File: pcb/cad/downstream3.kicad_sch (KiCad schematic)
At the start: 14 parts, among them J801 USB_C_Receptacle, U801 ECMF02-2AMX6, U802 ECMF02-2AMX6, U803 ECMF02-2AMX6, U804 ECMF02-2AMX6, U805 ECMF02-2AMX6, U806 ECMF02-2AMX6, U807 CBTL02043A, U808 TUSB320, U809 PI3USB221E, U810 LM73100, U811 TPS25947xx

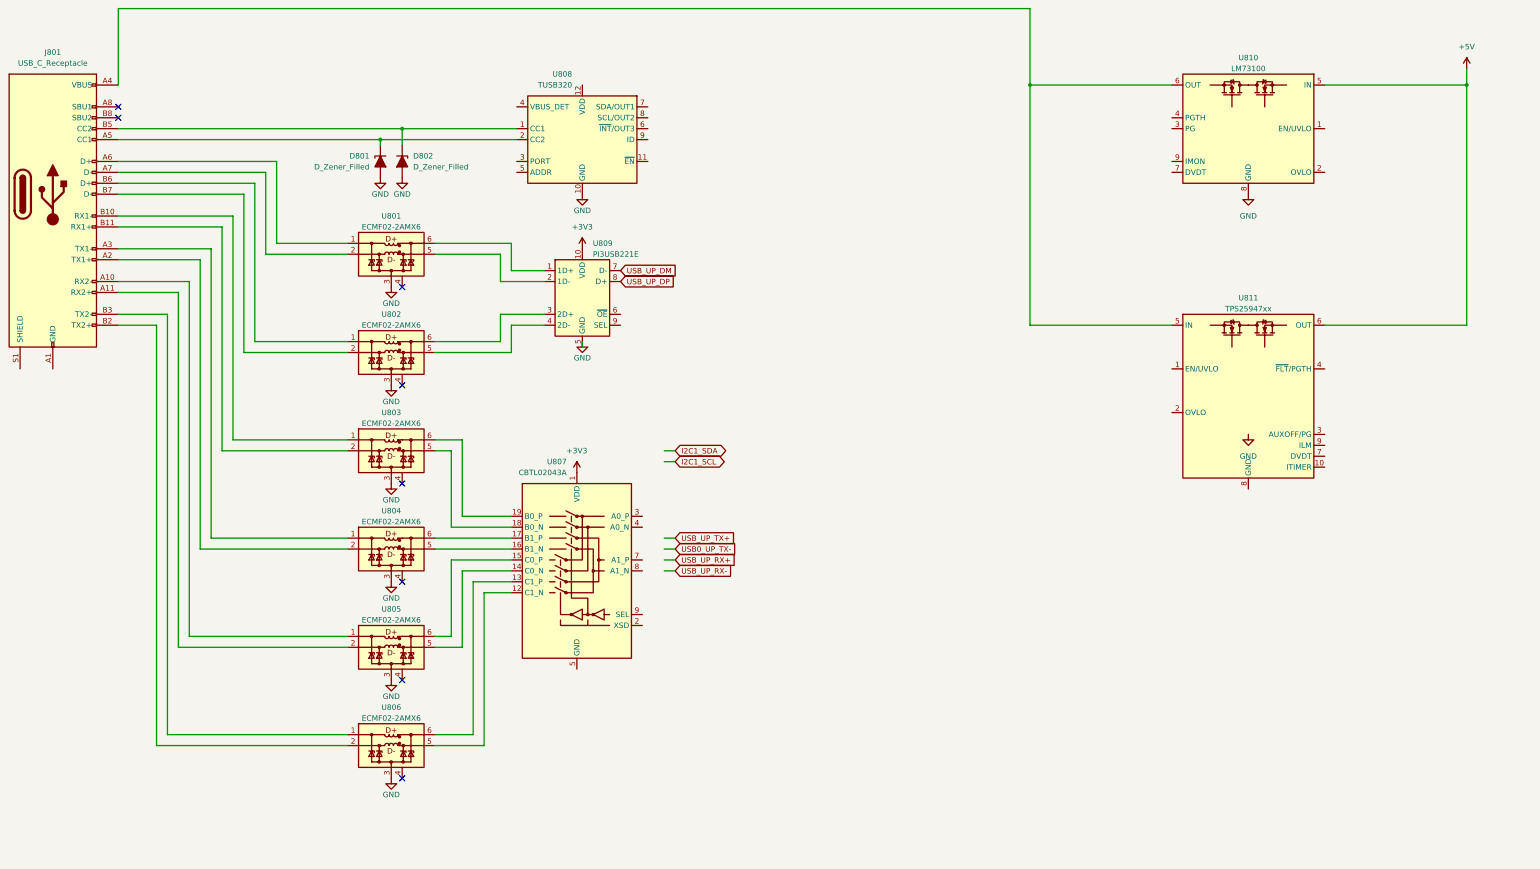
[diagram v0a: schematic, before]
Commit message: moved old-old-old backups and finished preliminary USB architecture
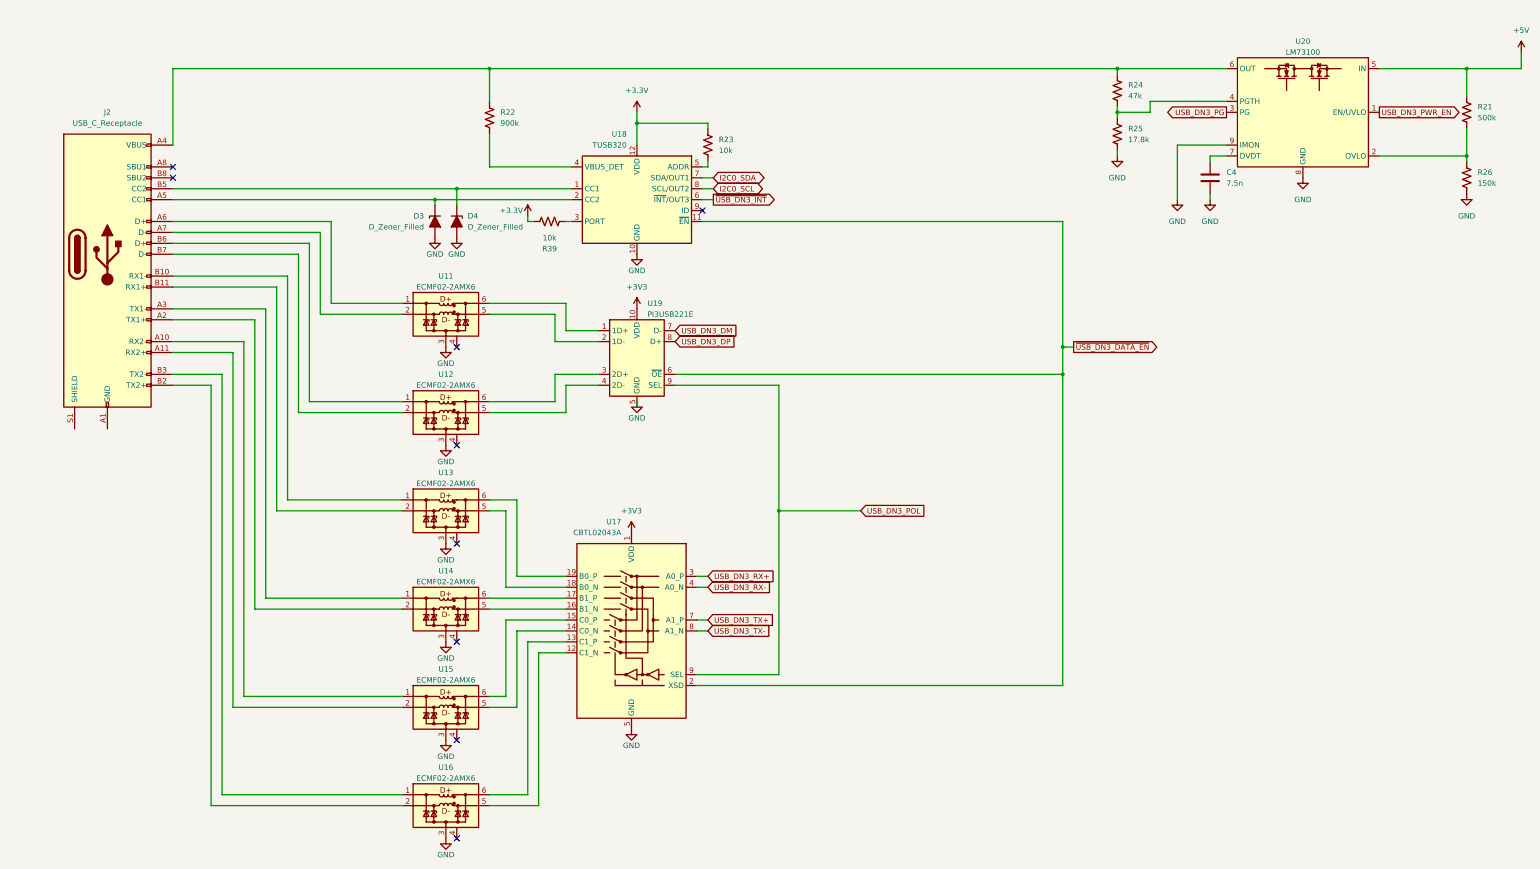
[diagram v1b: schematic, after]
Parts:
- removed D801, D802: D_Zener_Filled, symbol Device:D_Zener_Filled
- removed J801: USB_C_Receptacle, symbol Connector:USB_C_Receptacle
- removed U801, U802, U803, U804, U805, U806: ECMF02-2AMX6, Package_DFN_QFN:ST_UQFN-6L_1.5x1.7mm_P0.5mm, symbol Power_Protection:ECMF02-2AMX6
- removed U807: CBTL02043A, Package_DFN_QFN:WQFN-20-1EP_2.5x4.5mm_P0.5mm_EP1x2.9mm, symbol Analog_Switch:CBTL02043A
- removed U808: TUSB320, Package_DFN_QFN:Texas_X2QFN-12_1.6x1.6mm_P0.4mm, symbol Interface_USB:TUSB320
- removed U809: PI3USB221E, symbol Library:DIODES_PI3USB221E
- removed U810: LM73100, symbol Library:TI_LM73100
- removed U811: TPS25947xx, symbol Library:TI_TPS25947
- added C4: 7.5n, symbol Device:C
- added D3, D4: D_Zener_Filled, symbol Device:D_Zener_Filled
- added J2: USB_C_Receptacle, symbol Connector:USB_C_Receptacle
- added R21: 500k, symbol Device:R_US
- added R22: 900k, symbol Device:R_US
- added R23, R39: 10k, symbol Device:R_US
- added R24: 47k, symbol Device:R_US
- added R25: 17.8k, symbol Device:R_US
- added R26: 150k, symbol Device:R_US
- added U11, U12, U13, U14, U15, U16: ECMF02-2AMX6, Package_DFN_QFN:ST_UQFN-6L_1.5x1.7mm_P0.5mm, symbol Power_Protection:ECMF02-2AMX6
- added U17: CBTL02043A, Package_DFN_QFN:WQFN-20-1EP_2.5x4.5mm_P0.5mm_EP1x2.9mm, symbol Analog_Switch:CBTL02043A
- added U18: TUSB320, Package_DFN_QFN:Texas_X2QFN-12_1.6x1.6mm_P0.4mm, symbol Interface_USB:TUSB320
- added U19: PI3USB221E, symbol Library:DIODES_PI3USB221E
- added U20: LM73100, symbol Library:TI_LM73100
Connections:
- net +3V3: now also U17.1 (VDD), U17.10 (VDD), U17.6 (VDD), U19.10 (VDD)
- net +5V: now also R21.1, U20.5 (IN)
- net GND: now also C4.2, D3.2 (A), D4.2 (A), R25.2, R26.2, U11.3 (GND), U12.3 (GND), U13.3 (GND), U14.3 (GND), U15.3 (GND), U16.3 (GND), U17.11 (GND), U17.20 (GND), U17.21 (GND), U17.5 (GND), U18.10 (GND), U19.5 (GND), U20.8 (GND), U20.9 (IMON)
- new net: D4.1 (K), J2.B5 (CC2), U18.1 (CC1)
- new net: R24.2, R25.1, U20.4 (PGTH)
- new net: C4.1, U20.7 (DVDT)
- new net: J2.A3 (TX1-), U14.1 (D+_in)
- new net: J2.A2 (TX1+), U14.2 (D-_in)
- new net: U14.5 (D-_out), U17.16 (B1_N)
- new net: U14.6 (D+_out), U17.17 (B1_P)
- new net: J2.A6 (D+), U11.1 (D+_in)
- new net: J2.A7 (D-), U11.2 (D-_in)
- new net: U11.5 (D-_out), U19.2 (1D-)
- new net: U11.6 (D+_out), U19.1 (1D+)
- new net: J2.A10 (RX2-), U15.1 (D+_in)
- new net: J2.A11 (RX2+), U15.2 (D-_in)
- new net: U15.5 (D-_out), U17.14 (C0_N)
- new net: U15.6 (D+_out), U17.15 (C0_P)
- new net: J2.A4 (VBUS), J2.A9 (VBUS), J2.B4 (VBUS), J2.B9 (VBUS), R22.1, R24.1, U20.6 (OUT)
- new net: R22.2, U18.4 (VBUS_DET)
- new net: J2.B10 (RX1-), U13.1 (D+_in)
- new net: J2.B11 (RX1+), U13.2 (D-_in)
- new net: U13.5 (D-_out), U17.18 (B0_N)
- new net: U13.6 (D+_out), U17.19 (B0_P)
- new net: J2.B3 (TX2-), U16.1 (D+_in)
- new net: J2.B2 (TX2+), U16.2 (D-_in)
- new net: U16.5 (D-_out), U17.12 (C1_N)
- new net: U16.6 (D+_out), U17.13 (C1_P)
- new net: J2.A1 (GND), J2.A12 (GND), J2.B1 (GND), J2.B12 (GND)
- new net: D3.1 (K), J2.A5 (CC1), U18.2 (CC2)
- new net: J2.B6 (D+), U12.1 (D+_in)
- new net: J2.B7 (D-), U12.2 (D-_in)
- new net: R23.2, U18.5 (ADDR)
- new net: R21.2, R26.1, U20.2 (OVLO)
- new net: R39.1, U18.3 (PORT)
- new net: U12.6 (D+_out), U19.3 (2D+)
- new net: U12.5 (D-_out), U19.4 (2D-)
- new net +3.3V: R23.1, R39.2, U18.12 (VDD)
- new net I2C0_SCL: U18.8 (SCL/OUT2)
- new net I2C0_SDA: U18.7 (SDA/OUT1)
- new net USB_DN3_DM: U19.7 (D-)
- new net USB_DN3_DP: U19.8 (D+)
- new net USB_DN3_PG: U20.3 (PG)
- new net USB_DN3_POL: U17.9 (SEL), U19.9 (SEL)
- new net USB_DN3_PWR_EN: U20.1 (EN/UVLO)
- new net USB_DN3_RX+: U17.3 (A0_P)
- new net USB_DN3_RX-: U17.4 (A0_N)
- new net USB_DN3_TX+: U17.7 (A1_P)
- new net USB_DN3_TX-: U17.8 (A1_N)
- new net ~{USB_DN3_DATA_EN}: U17.2 (XSD), U18.11 (~{EN}), U19.6 (~{OE})
- new net ~{USB_DN3_INT}: U18.6 (~{INT}/OUT3)
- no-connect marks 8 -> 9
